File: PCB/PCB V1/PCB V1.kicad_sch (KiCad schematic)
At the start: 57 parts, among them J1 Screw_Terminal_01x03, J2 Screw_Terminal_01x03, J3 USB_B, J4 Conn_01x02_Pin, K1 Relay_SPDT, K2 Relay_SPDT, Q1 S8050, Q2 S8050, Q3 S8050, SW1 On/Off, SW2 SW_Push, SW3 SW_Push, U1 LM317_TO-220, U2 LM317_TO-220

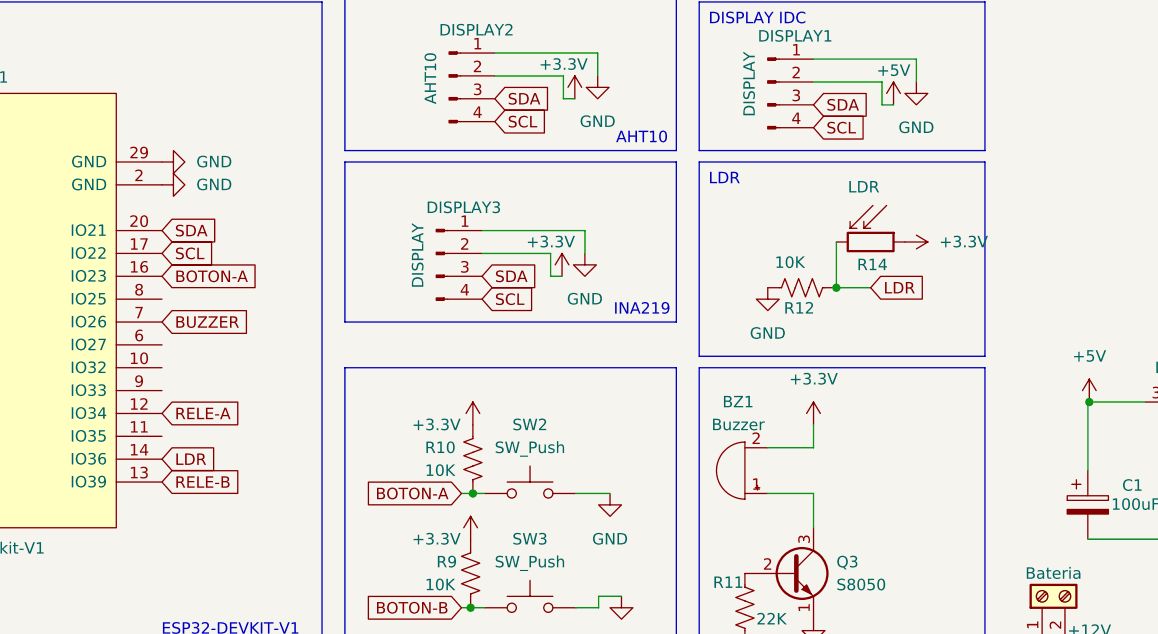
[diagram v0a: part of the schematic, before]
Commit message: .
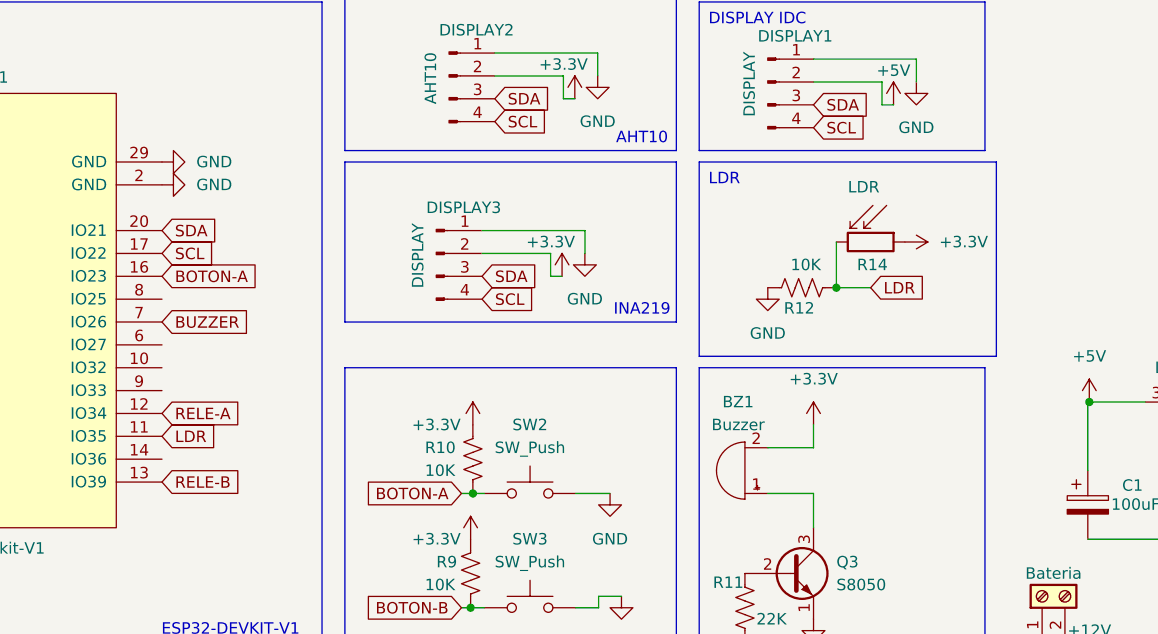
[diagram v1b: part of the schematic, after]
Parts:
- U1, U2: footprint Package_TO_SOT_THT:TO-220F-3_Vertical -> Package_TO_SOT_THT:TO-92_Inline
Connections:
- net LDR: now also ESP-1.11 (IO35); no longer ESP-1.14 (IO36)
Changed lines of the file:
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@@
 		(exclude_from_sim no)
 		(at 180.34 38.1 0)
-		(size 31.75 21.59)
+		(size 33.02 21.59)
 		(stroke
 			(width 0)
@@
 	(global_label "LDR"
 		(shape input)
-		(at 120.65 71.12 0)
+		(at 120.65 68.58 0)
 		(fields_autoplaced yes)
 		(effects
@@
 		)
 		(property "Intersheetrefs" "${INTERSHEET_REFS}"
-			(at 127.2033 71.12 0)
+			(at 127.2033 68.58 0)
 			(effects
 				(font
@@
 		)
 		(property "Value" "10K"
-			(at 188.722 49.276 90)
+			(at 190.5 49.53 90)
 			(effects
 				(font
@@
 			)
 		)
-		(property "Footprint" "Package_TO_SOT_THT:TO-220F-3_Vertical"
+		(property "Footprint" "Package_TO_SOT_THT:TO-92_Inline"
 			(at 237.49 58.42 0)
 			(effects
@@
 			)
 		)
-		(property "Footprint" "Package_TO_SOT_THT:TO-220F-3_Vertical"
+		(property "Footprint" "Package_TO_SOT_THT:TO-92_Inline"
 			(at 237.49 88.9 0)
 			(effects

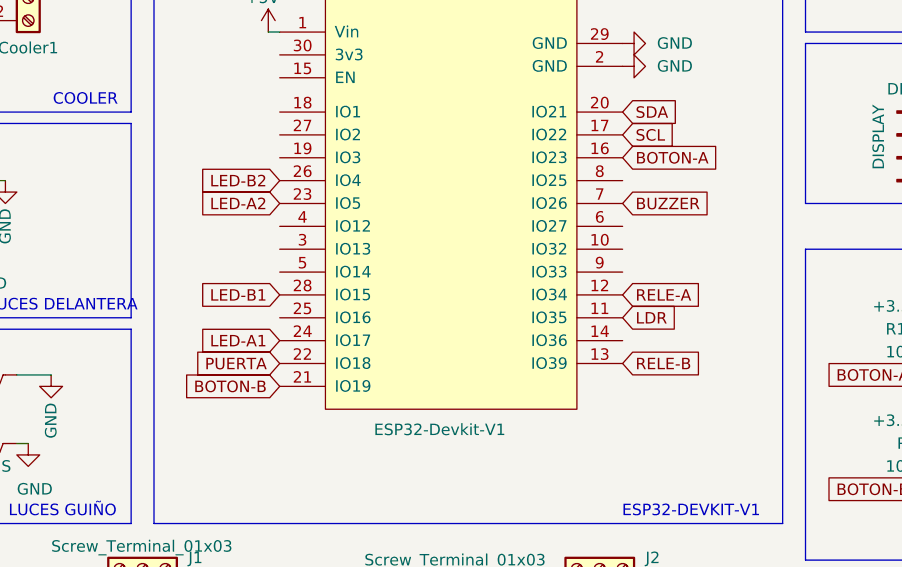
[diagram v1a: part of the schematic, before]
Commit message: .
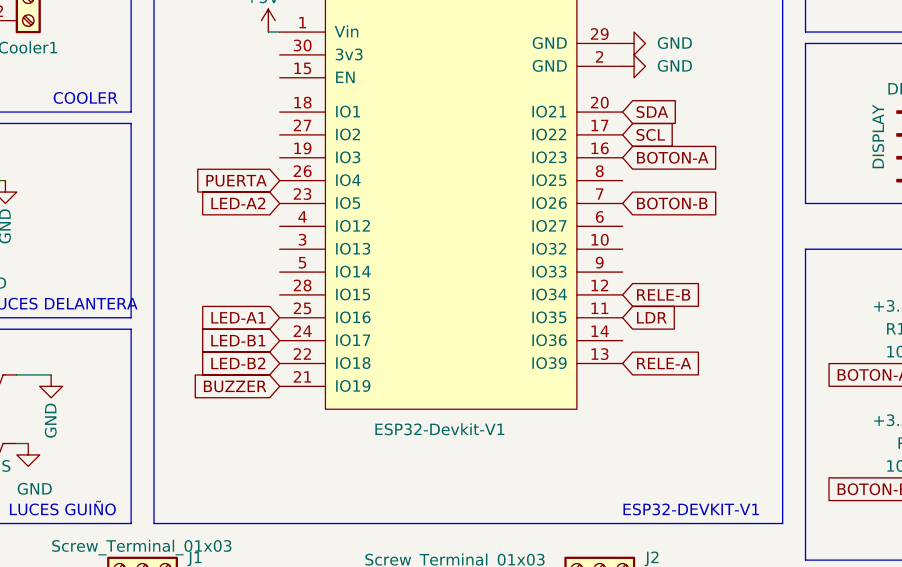
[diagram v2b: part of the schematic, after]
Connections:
- net BOTON-B: now also ESP-1.7 (IO26); no longer ESP-1.21 (IO19)
- net BUZZER: now also ESP-1.21 (IO19); no longer ESP-1.7 (IO26)
- net LED-A1: now also ESP-1.25 (IO16); no longer ESP-1.24 (IO17)
- net LED-B1: now also ESP-1.24 (IO17); no longer ESP-1.28 (IO15)
- net LED-B2: now also ESP-1.22 (IO18); no longer ESP-1.26 (IO4)
- net PUERTA: now also ESP-1.26 (IO4); no longer ESP-1.22 (IO18)
- net RELE-A: now also ESP-1.13 (IO39); no longer ESP-1.12 (IO34)
- net RELE-B: now also ESP-1.12 (IO34); no longer ESP-1.13 (IO39)

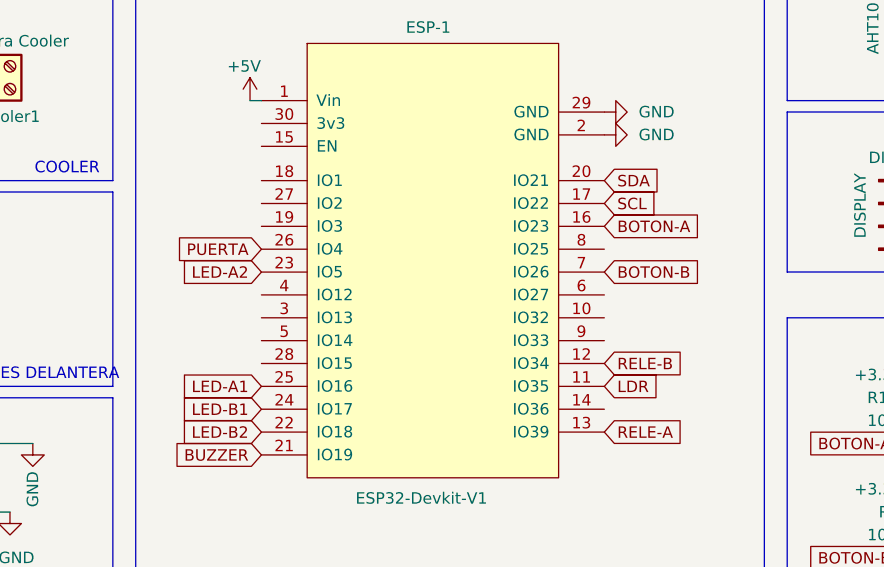
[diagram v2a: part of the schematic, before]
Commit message: .
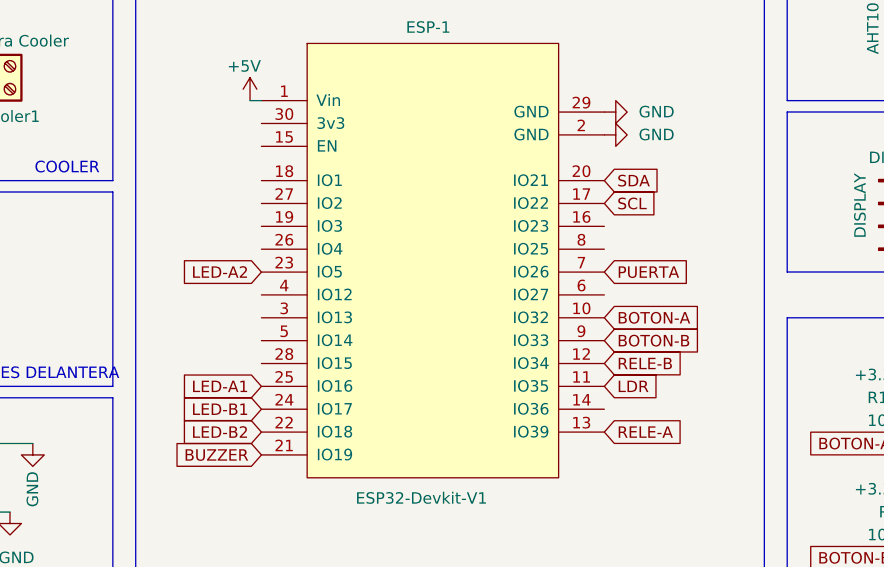
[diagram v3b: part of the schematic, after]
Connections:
- net BOTON-A: now also ESP-1.10 (IO32); no longer ESP-1.16 (IO23)
- net BOTON-B: now also ESP-1.9 (IO33); no longer ESP-1.7 (IO26)
- net PUERTA: now also ESP-1.7 (IO26); no longer ESP-1.26 (IO4)

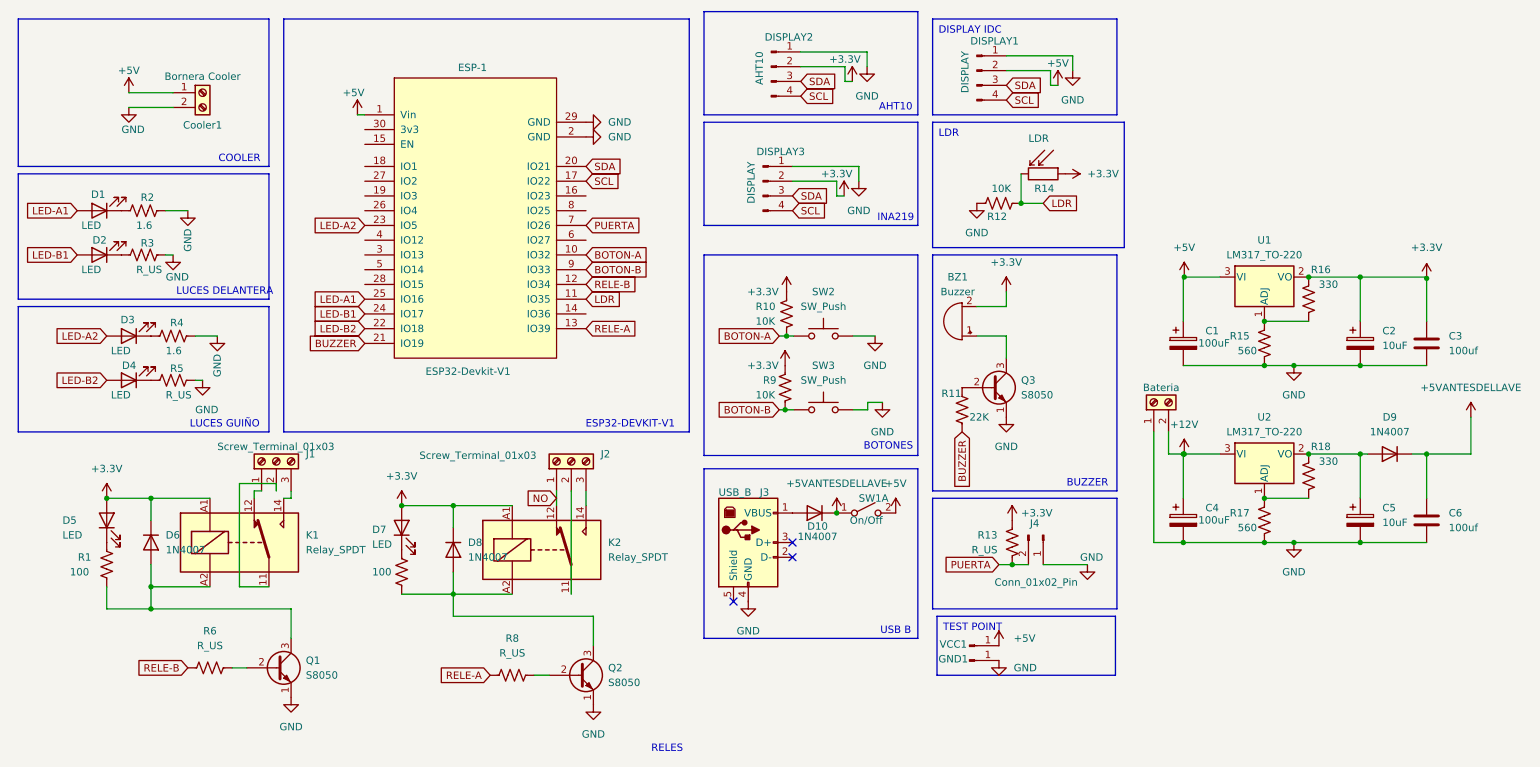
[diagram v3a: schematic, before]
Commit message: .
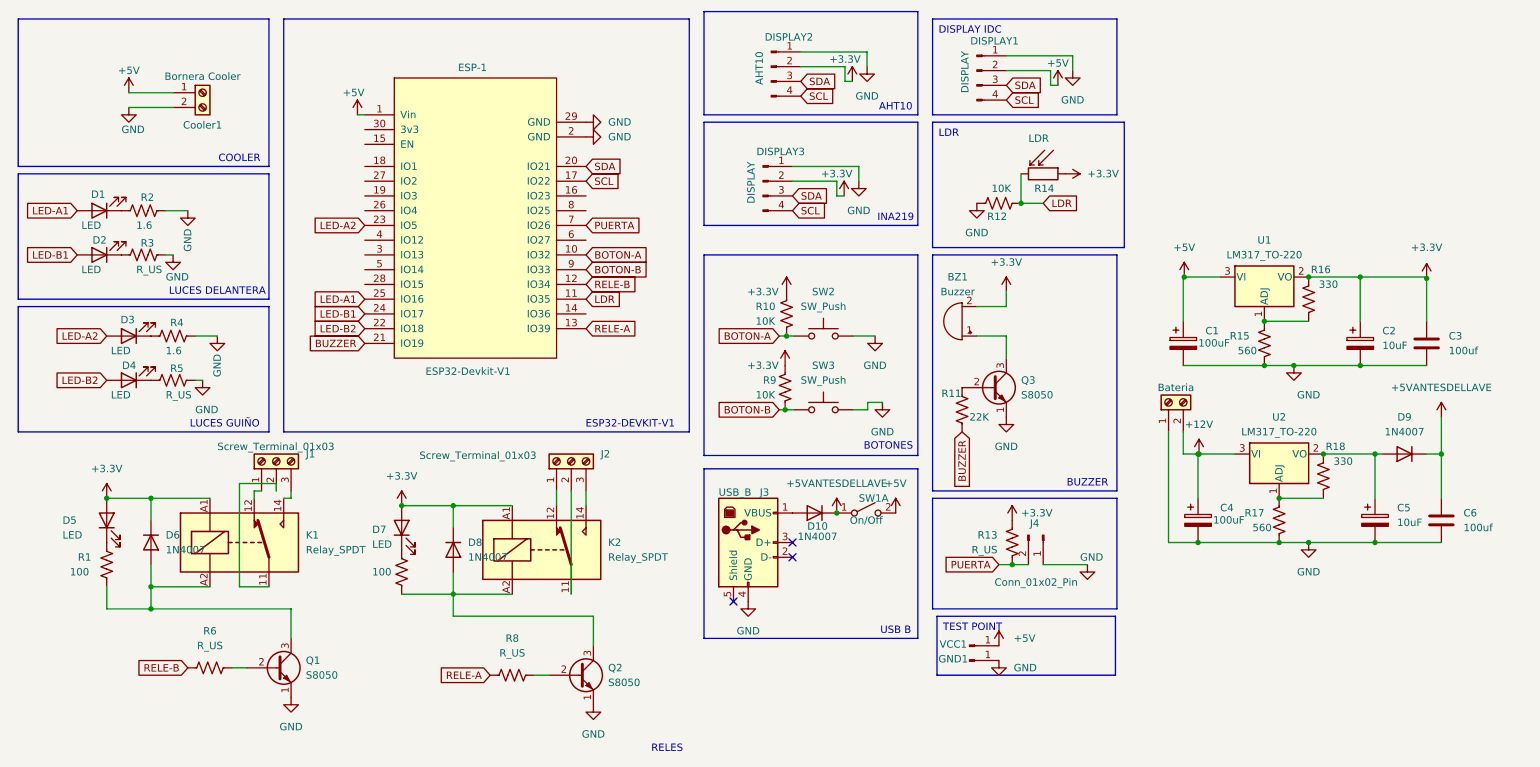
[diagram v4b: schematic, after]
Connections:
- net NO: no longer names the net of J2.1 (Pin_1), K2.12
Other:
- moved on the sheet: C4, C5, C6, D9, R17, R18, U2
